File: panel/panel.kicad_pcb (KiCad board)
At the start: 2 copper layers, 40 x 40 mm, 0 parts

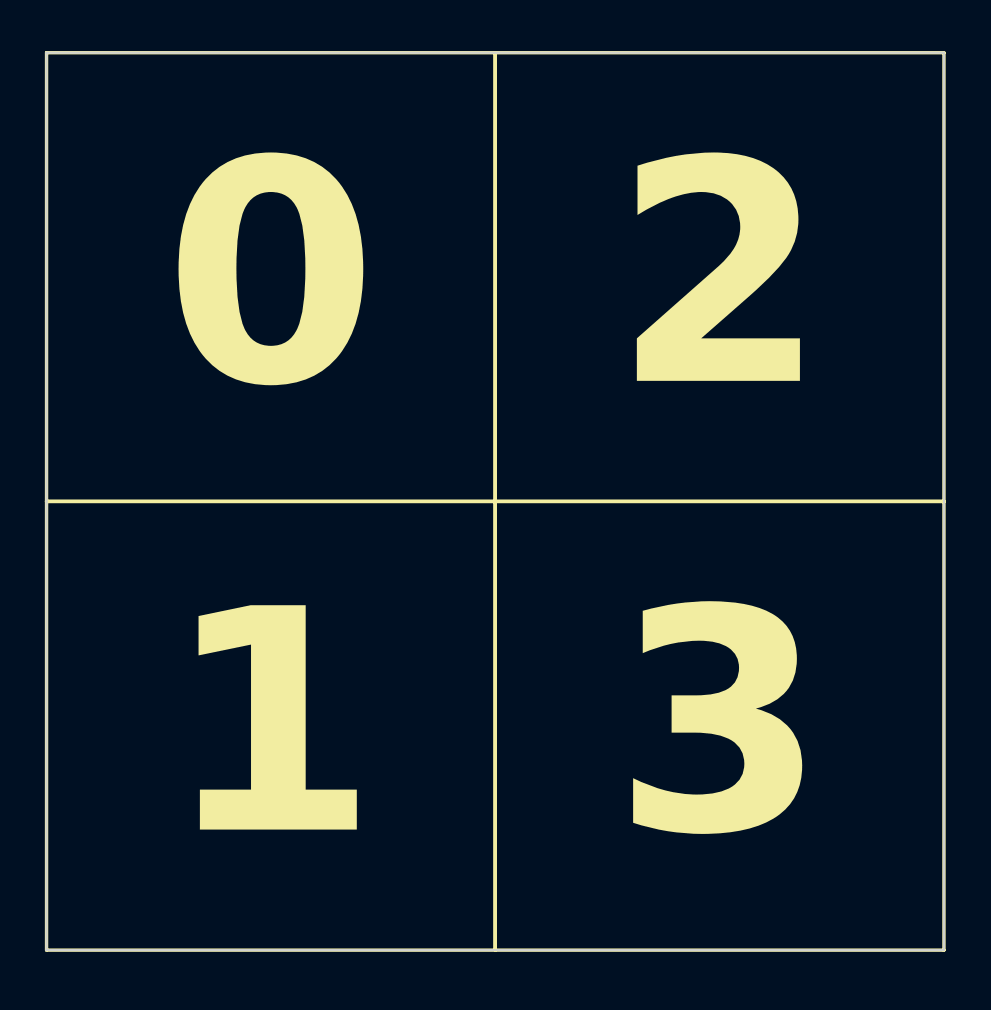
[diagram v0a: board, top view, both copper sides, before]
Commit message: Update panel
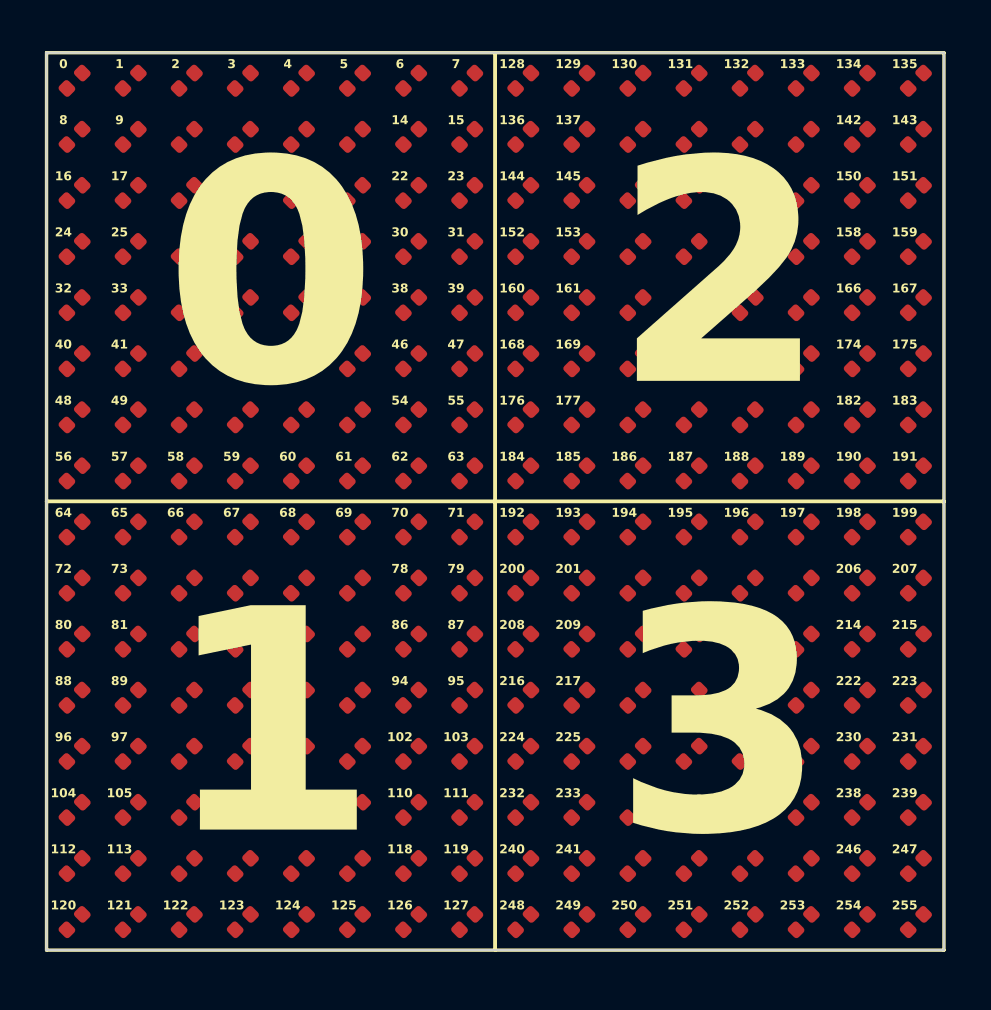
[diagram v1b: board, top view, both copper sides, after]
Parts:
- added REF**: LED_0402_1005Metric, LED_SMD:LED_0402_1005Metric, F.Cu at (146.2, 91.2)
- added REF**: LED_0402_1005Metric, LED_SMD:LED_0402_1005Metric, F.Cu at (138.8, 96.2)
- added REF**: LED_0402_1005Metric, LED_SMD:LED_0402_1005Metric, F.Cu at (116.2, 128.8)
- added REF**: LED_0402_1005Metric, LED_SMD:LED_0402_1005Metric, F.Cu at (116.2, 101.2)
- added REF**: LED_0402_1005Metric, LED_SMD:LED_0402_1005Metric, F.Cu at (153.8, 126.2)
- added REF**: LED_0402_1005Metric, LED_SMD:LED_0402_1005Metric, F.Cu at (151.2, 96.2)
- added REF**: LED_0402_1005Metric, LED_SMD:LED_0402_1005Metric, F.Cu at (118.8, 111.2)
- added REF**: LED_0402_1005Metric, LED_SMD:LED_0402_1005Metric, F.Cu at (128.8, 106.2)
- added REF**: LED_0402_1005Metric, LED_SMD:LED_0402_1005Metric, F.Cu at (131.2, 106.2)
- added REF**: LED_0402_1005Metric, LED_SMD:LED_0402_1005Metric, F.Cu at (116.2, 91.2)
- added REF**: LED_0402_1005Metric, LED_SMD:LED_0402_1005Metric, F.Cu at (128.8, 103.8)
- added REF**: LED_0402_1005Metric, LED_SMD:LED_0402_1005Metric, F.Cu at (138.8, 103.8)
- added REF**: LED_0402_1005Metric, LED_SMD:LED_0402_1005Metric, F.Cu at (126.2, 113.8)
- added REF**: LED_0402_1005Metric, LED_SMD:LED_0402_1005Metric, F.Cu at (121.2, 91.2)
- added REF**: LED_0402_1005Metric, LED_SMD:LED_0402_1005Metric, F.Cu at (138.8, 121.2)
- added REF**: LED_0402_1005Metric, LED_SMD:LED_0402_1005Metric, F.Cu at (136.2, 96.2)
- added REF**: LED_0402_1005Metric, LED_SMD:LED_0402_1005Metric, F.Cu at (153.8, 96.2)
- added REF**: LED_0402_1005Metric, LED_SMD:LED_0402_1005Metric, F.Cu at (153.8, 93.8)
- added REF**: LED_0402_1005Metric, LED_SMD:LED_0402_1005Metric, F.Cu at (148.8, 118.8)
- added REF**: LED_0402_1005Metric, LED_SMD:LED_0402_1005Metric, F.Cu at (138.8, 111.2)
- added REF**: LED_0402_1005Metric, LED_SMD:LED_0402_1005Metric, F.Cu at (118.8, 106.2)
- added REF**: LED_0402_1005Metric, LED_SMD:LED_0402_1005Metric, F.Cu at (116.2, 106.2)
- added REF**: LED_0402_1005Metric, LED_SMD:LED_0402_1005Metric, F.Cu at (131.2, 118.8)
- added REF**: LED_0402_1005Metric, LED_SMD:LED_0402_1005Metric, F.Cu at (136.2, 106.2)
- added REF**: LED_0402_1005Metric, LED_SMD:LED_0402_1005Metric, F.Cu at (128.8, 108.8)
- added REF**: LED_0402_1005Metric, LED_SMD:LED_0402_1005Metric, F.Cu at (143.8, 91.2)
- added REF**: LED_0402_1005Metric, LED_SMD:LED_0402_1005Metric, F.Cu at (128.8, 126.2)
- added REF**: LED_0402_1005Metric, LED_SMD:LED_0402_1005Metric, F.Cu at (126.2, 121.2)
- added REF**: LED_0402_1005Metric, LED_SMD:LED_0402_1005Metric, F.Cu at (131.2, 123.8)
- added REF**: LED_0402_1005Metric, LED_SMD:LED_0402_1005Metric, F.Cu at (148.8, 123.8)
- added REF**: LED_0402_1005Metric, LED_SMD:LED_0402_1005Metric, F.Cu at (131.2, 116.2)
- added REF**: LED_0402_1005Metric, LED_SMD:LED_0402_1005Metric, F.Cu at (141.2, 126.2)
- added REF**: LED_0402_1005Metric, LED_SMD:LED_0402_1005Metric, F.Cu at (128.8, 93.8)
- added REF**: LED_0402_1005Metric, LED_SMD:LED_0402_1005Metric, F.Cu at (136.2, 101.2)
- added REF**: LED_0402_1005Metric, LED_SMD:LED_0402_1005Metric, F.Cu at (131.2, 93.8)
- added REF**: LED_0402_1005Metric, LED_SMD:LED_0402_1005Metric, F.Cu at (128.8, 91.2)
- added REF**: LED_0402_1005Metric, LED_SMD:LED_0402_1005Metric, F.Cu at (118.8, 118.8)
- added REF**: LED_0402_1005Metric, LED_SMD:LED_0402_1005Metric, F.Cu at (128.8, 123.8)
- added REF**: LED_0402_1005Metric, LED_SMD:LED_0402_1005Metric, F.Cu at (136.2, 128.8)
- added REF**: LED_0402_1005Metric, LED_SMD:LED_0402_1005Metric, F.Cu at (116.2, 93.8)
- added REF**: LED_0402_1005Metric, LED_SMD:LED_0402_1005Metric, F.Cu at (133.8, 121.2)
- added REF**: LED_0402_1005Metric, LED_SMD:LED_0402_1005Metric, F.Cu at (123.8, 116.2)
- added REF**: LED_0402_1005Metric, LED_SMD:LED_0402_1005Metric, F.Cu at (118.8, 121.2)
- added REF**: LED_0402_1005Metric, LED_SMD:LED_0402_1005Metric, F.Cu at (126.2, 118.8)
- added REF**: LED_0402_1005Metric, LED_SMD:LED_0402_1005Metric, F.Cu at (148.8, 101.2)
- added REF**: LED_0402_1005Metric, LED_SMD:LED_0402_1005Metric, F.Cu at (118.8, 91.2)
- added REF**: LED_0402_1005Metric, LED_SMD:LED_0402_1005Metric, F.Cu at (141.2, 101.2)
- added REF**: LED_0402_1005Metric, LED_SMD:LED_0402_1005Metric, F.Cu at (143.8, 121.2)
- added REF**: LED_0402_1005Metric, LED_SMD:LED_0402_1005Metric, F.Cu at (128.8, 101.2)
- added REF**: LED_0402_1005Metric, LED_SMD:LED_0402_1005Metric, F.Cu at (143.8, 111.2)
- added REF**: LED_0402_1005Metric, LED_SMD:LED_0402_1005Metric, F.Cu at (148.8, 108.8)
- added REF**: LED_0402_1005Metric, LED_SMD:LED_0402_1005Metric, F.Cu at (121.2, 116.2)
- added REF**: LED_0402_1005Metric, LED_SMD:LED_0402_1005Metric, F.Cu at (153.8, 121.2)
- added REF**: LED_0402_1005Metric, LED_SMD:LED_0402_1005Metric, F.Cu at (126.2, 93.8)
- added REF**: LED_0402_1005Metric, LED_SMD:LED_0402_1005Metric, F.Cu at (118.8, 93.8)
- added REF**: LED_0402_1005Metric, LED_SMD:LED_0402_1005Metric, F.Cu at (143.8, 128.8)
- added REF**: LED_0402_1005Metric, LED_SMD:LED_0402_1005Metric, F.Cu at (133.8, 108.8)
- added REF**: LED_0402_1005Metric, LED_SMD:LED_0402_1005Metric, F.Cu at (138.8, 123.8)
- added REF**: LED_0402_1005Metric, LED_SMD:LED_0402_1005Metric, F.Cu at (123.8, 103.8)
- added REF**: LED_0402_1005Metric, LED_SMD:LED_0402_1005Metric, F.Cu at (138.8, 128.8)
- added REF**: LED_0402_1005Metric, LED_SMD:LED_0402_1005Metric, F.Cu at (131.2, 98.8)
- added REF**: LED_0402_1005Metric, LED_SMD:LED_0402_1005Metric, F.Cu at (126.2, 111.2)
- added REF**: LED_0402_1005Metric, LED_SMD:LED_0402_1005Metric, F.Cu at (153.8, 111.2)
- added REF**: LED_0402_1005Metric, LED_SMD:LED_0402_1005Metric, F.Cu at (153.8, 113.8)
- added REF**: LED_0402_1005Metric, LED_SMD:LED_0402_1005Metric, F.Cu at (148.8, 126.2)
- added REF**: LED_0402_1005Metric, LED_SMD:LED_0402_1005Metric, F.Cu at (133.8, 103.8)
- added REF**: LED_0402_1005Metric, LED_SMD:LED_0402_1005Metric, F.Cu at (133.8, 96.2)
- added REF**: LED_0402_1005Metric, LED_SMD:LED_0402_1005Metric, F.Cu at (131.2, 108.8)
- added REF**: LED_0402_1005Metric, LED_SMD:LED_0402_1005Metric, F.Cu at (136.2, 111.2)
- added REF**: LED_0402_1005Metric, LED_SMD:LED_0402_1005Metric, F.Cu at (121.2, 113.8)
- added REF**: LED_0402_1005Metric, LED_SMD:LED_0402_1005Metric, F.Cu at (141.2, 106.2)
- added REF**: LED_0402_1005Metric, LED_SMD:LED_0402_1005Metric, F.Cu at (128.8, 128.8)
- added REF**: LED_0402_1005Metric, LED_SMD:LED_0402_1005Metric, F.Cu at (146.2, 103.8)
- added REF**: LED_0402_1005Metric, LED_SMD:LED_0402_1005Metric, F.Cu at (141.2, 121.2)
- added REF**: LED_0402_1005Metric, LED_SMD:LED_0402_1005Metric, F.Cu at (146.2, 106.2)
- added REF**: LED_0402_1005Metric, LED_SMD:LED_0402_1005Metric, F.Cu at (153.8, 123.8)
- added REF**: LED_0402_1005Metric, LED_SMD:LED_0402_1005Metric, F.Cu at (118.8, 113.8)
- added REF**: LED_0402_1005Metric, LED_SMD:LED_0402_1005Metric, F.Cu at (153.8, 98.8)
- added REF**: LED_0402_1005Metric, LED_SMD:LED_0402_1005Metric, F.Cu at (143.8, 98.8)
- added REF**: LED_0402_1005Metric, LED_SMD:LED_0402_1005Metric, F.Cu at (116.2, 96.2)
- added REF**: LED_0402_1005Metric, LED_SMD:LED_0402_1005Metric, F.Cu at (138.8, 98.8)
- added REF**: LED_0402_1005Metric, LED_SMD:LED_0402_1005Metric, F.Cu at (118.8, 116.2)
- added REF**: LED_0402_1005Metric, LED_SMD:LED_0402_1005Metric, F.Cu at (143.8, 103.8)
- added REF**: LED_0402_1005Metric, LED_SMD:LED_0402_1005Metric, F.Cu at (126.2, 128.8)
- added REF**: LED_0402_1005Metric, LED_SMD:LED_0402_1005Metric, F.Cu at (138.8, 113.8)
- added REF**: LED_0402_1005Metric, LED_SMD:LED_0402_1005Metric, F.Cu at (133.8, 113.8)
- added REF**: LED_0402_1005Metric, LED_SMD:LED_0402_1005Metric, F.Cu at (118.8, 101.2)
- added REF**: LED_0402_1005Metric, LED_SMD:LED_0402_1005Metric, F.Cu at (138.8, 93.8)
- added REF**: LED_0402_1005Metric, LED_SMD:LED_0402_1005Metric, F.Cu at (131.2, 113.8)
- added REF**: LED_0402_1005Metric, LED_SMD:LED_0402_1005Metric, F.Cu at (116.2, 111.2)
- added REF**: LED_0402_1005Metric, LED_SMD:LED_0402_1005Metric, F.Cu at (126.2, 96.2)
- added REF**: LED_0402_1005Metric, LED_SMD:LED_0402_1005Metric, F.Cu at (118.8, 108.8)
- added REF**: LED_0402_1005Metric, LED_SMD:LED_0402_1005Metric, F.Cu at (126.2, 116.2)
- added REF**: LED_0402_1005Metric, LED_SMD:LED_0402_1005Metric, F.Cu at (143.8, 106.2)
- added REF**: LED_0402_1005Metric, LED_SMD:LED_0402_1005Metric, F.Cu at (116.2, 108.8)
- added REF**: LED_0402_1005Metric, LED_SMD:LED_0402_1005Metric, F.Cu at (136.2, 121.2)
- added REF**: LED_0402_1005Metric, LED_SMD:LED_0402_1005Metric, F.Cu at (121.2, 103.8)
- added REF**: LED_0402_1005Metric, LED_SMD:LED_0402_1005Metric, F.Cu at (138.8, 108.8)
- added REF**: LED_0402_1005Metric, LED_SMD:LED_0402_1005Metric, F.Cu at (133.8, 93.8)
- added REF**: LED_0402_1005Metric, LED_SMD:LED_0402_1005Metric, F.Cu at (148.8, 93.8)
- added REF**: LED_0402_1005Metric, LED_SMD:LED_0402_1005Metric, F.Cu at (116.2, 126.2)
- added REF**: LED_0402_1005Metric, LED_SMD:LED_0402_1005Metric, F.Cu at (146.2, 101.2)
- added REF**: LED_0402_1005Metric, LED_SMD:LED_0402_1005Metric, F.Cu at (123.8, 123.8)
- added REF**: LED_0402_1005Metric, LED_SMD:LED_0402_1005Metric, F.Cu at (121.2, 126.2)
- added REF**: LED_0402_1005Metric, LED_SMD:LED_0402_1005Metric, F.Cu at (148.8, 116.2)
- added REF**: LED_0402_1005Metric, LED_SMD:LED_0402_1005Metric, F.Cu at (116.2, 123.8)
- added REF**: LED_0402_1005Metric, LED_SMD:LED_0402_1005Metric, F.Cu at (131.2, 126.2)
- added REF**: LED_0402_1005Metric, LED_SMD:LED_0402_1005Metric, F.Cu at (131.2, 96.2)
- added REF**: LED_0402_1005Metric, LED_SMD:LED_0402_1005Metric, F.Cu at (118.8, 123.8)
- added REF**: LED_0402_1005Metric, LED_SMD:LED_0402_1005Metric, F.Cu at (138.8, 106.2)
- added REF**: LED_0402_1005Metric, LED_SMD:LED_0402_1005Metric, F.Cu at (141.2, 96.2)
- added REF**: LED_0402_1005Metric, LED_SMD:LED_0402_1005Metric, F.Cu at (153.8, 116.2)
- added REF**: LED_0402_1005Metric, LED_SMD:LED_0402_1005Metric, F.Cu at (118.8, 126.2)
- added REF**: LED_0402_1005Metric, LED_SMD:LED_0402_1005Metric, F.Cu at (151.2, 123.8)
- added REF**: LED_0402_1005Metric, LED_SMD:LED_0402_1005Metric, F.Cu at (133.8, 128.8)
- added REF**: LED_0402_1005Metric, LED_SMD:LED_0402_1005Metric, F.Cu at (143.8, 116.2)
- added REF**: LED_0402_1005Metric, LED_SMD:LED_0402_1005Metric, F.Cu at (128.8, 98.8)
- added REF**: LED_0402_1005Metric, LED_SMD:LED_0402_1005Metric, F.Cu at (141.2, 118.8)
- added REF**: LED_0402_1005Metric, LED_SMD:LED_0402_1005Metric, F.Cu at (148.8, 121.2)
- added REF**: LED_0402_1005Metric, LED_SMD:LED_0402_1005Metric, F.Cu at (141.2, 116.2)
- added REF**: LED_0402_1005Metric, LED_SMD:LED_0402_1005Metric, F.Cu at (141.2, 98.8)
- added REF**: LED_0402_1005Metric, LED_SMD:LED_0402_1005Metric, F.Cu at (136.2, 126.2)
- added REF**: LED_0402_1005Metric, LED_SMD:LED_0402_1005Metric, F.Cu at (136.2, 108.8)
- added REF**: LED_0402_1005Metric, LED_SMD:LED_0402_1005Metric, F.Cu at (116.2, 121.2)
- added REF**: LED_0402_1005Metric, LED_SMD:LED_0402_1005Metric, F.Cu at (141.2, 111.2)
- added REF**: LED_0402_1005Metric, LED_SMD:LED_0402_1005Metric, F.Cu at (126.2, 103.8)
- added REF**: LED_0402_1005Metric, LED_SMD:LED_0402_1005Metric, F.Cu at (146.2, 108.8)
- added REF**: LED_0402_1005Metric, LED_SMD:LED_0402_1005Metric, F.Cu at (143.8, 113.8)
- added REF**: LED_0402_1005Metric, LED_SMD:LED_0402_1005Metric, F.Cu at (146.2, 126.2)
- added REF**: LED_0402_1005Metric, LED_SMD:LED_0402_1005Metric, F.Cu at (121.2, 108.8)
- added REF**: LED_0402_1005Metric, LED_SMD:LED_0402_1005Metric, F.Cu at (126.2, 123.8)
- added REF**: LED_0402_1005Metric, LED_SMD:LED_0402_1005Metric, F.Cu at (123.8, 106.2)
- added REF**: LED_0402_1005Metric, LED_SMD:LED_0402_1005Metric, F.Cu at (121.2, 118.8)
- added REF**: LED_0402_1005Metric, LED_SMD:LED_0402_1005Metric, F.Cu at (131.2, 101.2)
- added REF**: LED_0402_1005Metric, LED_SMD:LED_0402_1005Metric, F.Cu at (131.2, 111.2)
- added REF**: LED_0402_1005Metric, LED_SMD:LED_0402_1005Metric, F.Cu at (126.2, 106.2)
- added REF**: LED_0402_1005Metric, LED_SMD:LED_0402_1005Metric, F.Cu at (128.8, 96.2)
- added REF**: LED_0402_1005Metric, LED_SMD:LED_0402_1005Metric, F.Cu at (136.2, 103.8)
- added REF**: LED_0402_1005Metric, LED_SMD:LED_0402_1005Metric, F.Cu at (126.2, 108.8)
- added REF**: LED_0402_1005Metric, LED_SMD:LED_0402_1005Metric, F.Cu at (153.8, 106.2)
- added REF**: LED_0402_1005Metric, LED_SMD:LED_0402_1005Metric, F.Cu at (143.8, 93.8)
- added REF**: LED_0402_1005Metric, LED_SMD:LED_0402_1005Metric, F.Cu at (118.8, 96.2)
- added REF**: LED_0402_1005Metric, LED_SMD:LED_0402_1005Metric, F.Cu at (151.2, 113.8)
- added REF**: LED_0402_1005Metric, LED_SMD:LED_0402_1005Metric, F.Cu at (146.2, 123.8)
- added REF**: LED_0402_1005Metric, LED_SMD:LED_0402_1005Metric, F.Cu at (151.2, 101.2)
- added REF**: LED_0402_1005Metric, LED_SMD:LED_0402_1005Metric, F.Cu at (141.2, 123.8)
- added REF**: LED_0402_1005Metric, LED_SMD:LED_0402_1005Metric, F.Cu at (128.8, 116.2)
- added REF**: LED_0402_1005Metric, LED_SMD:LED_0402_1005Metric, F.Cu at (153.8, 128.8)
- added REF**: LED_0402_1005Metric, LED_SMD:LED_0402_1005Metric, F.Cu at (151.2, 108.8)
- added REF**: LED_0402_1005Metric, LED_SMD:LED_0402_1005Metric, F.Cu at (133.8, 91.2)
- added REF**: LED_0402_1005Metric, LED_SMD:LED_0402_1005Metric, F.Cu at (148.8, 111.2)
- added REF**: LED_0402_1005Metric, LED_SMD:LED_0402_1005Metric, F.Cu at (148.8, 128.8)
- added REF**: LED_0402_1005Metric, LED_SMD:LED_0402_1005Metric, F.Cu at (153.8, 91.2)
- added REF**: LED_0402_1005Metric, LED_SMD:LED_0402_1005Metric, F.Cu at (148.8, 106.2)
- added REF**: LED_0402_1005Metric, LED_SMD:LED_0402_1005Metric, F.Cu at (143.8, 123.8)
- added REF**: LED_0402_1005Metric, LED_SMD:LED_0402_1005Metric, F.Cu at (141.2, 113.8)
- added REF**: LED_0402_1005Metric, LED_SMD:LED_0402_1005Metric, F.Cu at (126.2, 98.8)
- added REF**: LED_0402_1005Metric, LED_SMD:LED_0402_1005Metric, F.Cu at (131.2, 103.8)
- added REF**: LED_0402_1005Metric, LED_SMD:LED_0402_1005Metric, F.Cu at (116.2, 103.8)
- added REF**: LED_0402_1005Metric, LED_SMD:LED_0402_1005Metric, F.Cu at (123.8, 91.2)
- added REF**: LED_0402_1005Metric, LED_SMD:LED_0402_1005Metric, F.Cu at (116.2, 116.2)
- added REF**: LED_0402_1005Metric, LED_SMD:LED_0402_1005Metric, F.Cu at (138.8, 126.2)
- added REF**: LED_0402_1005Metric, LED_SMD:LED_0402_1005Metric, F.Cu at (146.2, 98.8)
- added REF**: LED_0402_1005Metric, LED_SMD:LED_0402_1005Metric, F.Cu at (136.2, 118.8)
- added REF**: LED_0402_1005Metric, LED_SMD:LED_0402_1005Metric, F.Cu at (148.8, 113.8)
- added REF**: LED_0402_1005Metric, LED_SMD:LED_0402_1005Metric, F.Cu at (151.2, 128.8)
- added REF**: LED_0402_1005Metric, LED_SMD:LED_0402_1005Metric, F.Cu at (136.2, 98.8)
- added REF**: LED_0402_1005Metric, LED_SMD:LED_0402_1005Metric, F.Cu at (123.8, 101.2)
- added REF**: LED_0402_1005Metric, LED_SMD:LED_0402_1005Metric, F.Cu at (136.2, 116.2)
- added REF**: LED_0402_1005Metric, LED_SMD:LED_0402_1005Metric, F.Cu at (153.8, 108.8)
- added REF**: LED_0402_1005Metric, LED_SMD:LED_0402_1005Metric, F.Cu at (146.2, 116.2)
- added REF**: LED_0402_1005Metric, LED_SMD:LED_0402_1005Metric, F.Cu at (138.8, 101.2)
- added REF**: LED_0402_1005Metric, LED_SMD:LED_0402_1005Metric, F.Cu at (153.8, 118.8)
- added REF**: LED_0402_1005Metric, LED_SMD:LED_0402_1005Metric, F.Cu at (123.8, 111.2)
- added REF**: LED_0402_1005Metric, LED_SMD:LED_0402_1005Metric, F.Cu at (146.2, 93.8)
- added REF**: LED_0402_1005Metric, LED_SMD:LED_0402_1005Metric, F.Cu at (136.2, 91.2)
- added REF**: LED_0402_1005Metric, LED_SMD:LED_0402_1005Metric, F.Cu at (118.8, 98.8)
- added REF**: LED_0402_1005Metric, LED_SMD:LED_0402_1005Metric, F.Cu at (123.8, 96.2)
- added REF**: LED_0402_1005Metric, LED_SMD:LED_0402_1005Metric, F.Cu at (148.8, 91.2)
- added REF**: LED_0402_1005Metric, LED_SMD:LED_0402_1005Metric, F.Cu at (143.8, 96.2)
- added REF**: LED_0402_1005Metric, LED_SMD:LED_0402_1005Metric, F.Cu at (133.8, 111.2)
- added REF**: LED_0402_1005Metric, LED_SMD:LED_0402_1005Metric, F.Cu at (146.2, 113.8)
- added REF**: LED_0402_1005Metric, LED_SMD:LED_0402_1005Metric, F.Cu at (151.2, 91.2)
- added REF**: LED_0402_1005Metric, LED_SMD:LED_0402_1005Metric, F.Cu at (143.8, 101.2)
- added REF**: LED_0402_1005Metric, LED_SMD:LED_0402_1005Metric, F.Cu at (133.8, 106.2)
- added REF**: LED_0402_1005Metric, LED_SMD:LED_0402_1005Metric, F.Cu at (123.8, 121.2)
- added REF**: LED_0402_1005Metric, LED_SMD:LED_0402_1005Metric, F.Cu at (121.2, 93.8)
- added REF**: LED_0402_1005Metric, LED_SMD:LED_0402_1005Metric, F.Cu at (128.8, 111.2)
- added REF**: LED_0402_1005Metric, LED_SMD:LED_0402_1005Metric, F.Cu at (151.2, 118.8)
- added REF**: LED_0402_1005Metric, LED_SMD:LED_0402_1005Metric, F.Cu at (143.8, 118.8)
- added REF**: LED_0402_1005Metric, LED_SMD:LED_0402_1005Metric, F.Cu at (136.2, 113.8)
- added REF**: LED_0402_1005Metric, LED_SMD:LED_0402_1005Metric, F.Cu at (123.8, 113.8)
- added REF**: LED_0402_1005Metric, LED_SMD:LED_0402_1005Metric, F.Cu at (121.2, 123.8)
- added REF**: LED_0402_1005Metric, LED_SMD:LED_0402_1005Metric, F.Cu at (126.2, 91.2)
- added REF**: LED_0402_1005Metric, LED_SMD:LED_0402_1005Metric, F.Cu at (138.8, 91.2)
- added REF**: LED_0402_1005Metric, LED_SMD:LED_0402_1005Metric, F.Cu at (151.2, 98.8)
- added REF**: LED_0402_1005Metric, LED_SMD:LED_0402_1005Metric, F.Cu at (133.8, 118.8)
- added REF**: LED_0402_1005Metric, LED_SMD:LED_0402_1005Metric, F.Cu at (116.2, 118.8)
- added REF**: LED_0402_1005Metric, LED_SMD:LED_0402_1005Metric, F.Cu at (136.2, 93.8)
- added REF**: LED_0402_1005Metric, LED_SMD:LED_0402_1005Metric, F.Cu at (138.8, 118.8)
- added REF**: LED_0402_1005Metric, LED_SMD:LED_0402_1005Metric, F.Cu at (123.8, 128.8)
- added REF**: LED_0402_1005Metric, LED_SMD:LED_0402_1005Metric, F.Cu at (123.8, 98.8)
- added REF**: LED_0402_1005Metric, LED_SMD:LED_0402_1005Metric, F.Cu at (123.8, 126.2)
- added REF**: LED_0402_1005Metric, LED_SMD:LED_0402_1005Metric, F.Cu at (131.2, 121.2)
- added REF**: LED_0402_1005Metric, LED_SMD:LED_0402_1005Metric, F.Cu at (133.8, 116.2)
- added REF**: LED_0402_1005Metric, LED_SMD:LED_0402_1005Metric, F.Cu at (121.2, 121.2)
- added REF**: LED_0402_1005Metric, LED_SMD:LED_0402_1005Metric, F.Cu at (133.8, 101.2)
- added REF**: LED_0402_1005Metric, LED_SMD:LED_0402_1005Metric, F.Cu at (133.8, 126.2)
- added REF**: LED_0402_1005Metric, LED_SMD:LED_0402_1005Metric, F.Cu at (116.2, 98.8)
- added REF**: LED_0402_1005Metric, LED_SMD:LED_0402_1005Metric, F.Cu at (141.2, 93.8)
- added REF**: LED_0402_1005Metric, LED_SMD:LED_0402_1005Metric, F.Cu at (141.2, 103.8)
- added REF**: LED_0402_1005Metric, LED_SMD:LED_0402_1005Metric, F.Cu at (133.8, 123.8)
- added REF**: LED_0402_1005Metric, LED_SMD:LED_0402_1005Metric, F.Cu at (148.8, 98.8)
- added REF**: LED_0402_1005Metric, LED_SMD:LED_0402_1005Metric, F.Cu at (118.8, 103.8)
- added REF**: LED_0402_1005Metric, LED_SMD:LED_0402_1005Metric, F.Cu at (121.2, 128.8)
- added REF**: LED_0402_1005Metric, LED_SMD:LED_0402_1005Metric, F.Cu at (121.2, 111.2)
- added REF**: LED_0402_1005Metric, LED_SMD:LED_0402_1005Metric, F.Cu at (143.8, 108.8)
- added REF**: LED_0402_1005Metric, LED_SMD:LED_0402_1005Metric, F.Cu at (128.8, 118.8)
- added REF**: LED_0402_1005Metric, LED_SMD:LED_0402_1005Metric, F.Cu at (131.2, 128.8)
- added REF**: LED_0402_1005Metric, LED_SMD:LED_0402_1005Metric, F.Cu at (136.2, 123.8)
- added REF**: LED_0402_1005Metric, LED_SMD:LED_0402_1005Metric, F.Cu at (146.2, 96.2)
- added REF**: LED_0402_1005Metric, LED_SMD:LED_0402_1005Metric, F.Cu at (118.8, 128.8)
- added REF**: LED_0402_1005Metric, LED_SMD:LED_0402_1005Metric, F.Cu at (133.8, 98.8)
- added REF**: LED_0402_1005Metric, LED_SMD:LED_0402_1005Metric, F.Cu at (151.2, 103.8)
- added REF**: LED_0402_1005Metric, LED_SMD:LED_0402_1005Metric, F.Cu at (121.2, 96.2)
- added REF**: LED_0402_1005Metric, LED_SMD:LED_0402_1005Metric, F.Cu at (141.2, 128.8)
- added REF**: LED_0402_1005Metric, LED_SMD:LED_0402_1005Metric, F.Cu at (138.8, 116.2)
- added REF**: LED_0402_1005Metric, LED_SMD:LED_0402_1005Metric, F.Cu at (146.2, 128.8)
- added REF**: LED_0402_1005Metric, LED_SMD:LED_0402_1005Metric, F.Cu at (151.2, 93.8)
- added REF**: LED_0402_1005Metric, LED_SMD:LED_0402_1005Metric, F.Cu at (123.8, 118.8)
- added REF**: LED_0402_1005Metric, LED_SMD:LED_0402_1005Metric, F.Cu at (141.2, 108.8)
- added REF**: LED_0402_1005Metric, LED_SMD:LED_0402_1005Metric, F.Cu at (121.2, 101.2)
- added REF**: LED_0402_1005Metric, LED_SMD:LED_0402_1005Metric, F.Cu at (121.2, 98.8)
- added REF**: LED_0402_1005Metric, LED_SMD:LED_0402_1005Metric, F.Cu at (153.8, 101.2)
- added REF**: LED_0402_1005Metric, LED_SMD:LED_0402_1005Metric, F.Cu at (128.8, 113.8)
- added REF**: LED_0402_1005Metric, LED_SMD:LED_0402_1005Metric, F.Cu at (151.2, 111.2)
- added REF**: LED_0402_1005Metric, LED_SMD:LED_0402_1005Metric, F.Cu at (128.8, 121.2)
- added REF**: LED_0402_1005Metric, LED_SMD:LED_0402_1005Metric, F.Cu at (151.2, 126.2)
- added REF**: LED_0402_1005Metric, LED_SMD:LED_0402_1005Metric, F.Cu at (126.2, 101.2)
- added REF**: LED_0402_1005Metric, LED_SMD:LED_0402_1005Metric, F.Cu at (131.2, 91.2)
- added REF**: LED_0402_1005Metric, LED_SMD:LED_0402_1005Metric, F.Cu at (146.2, 111.2)
- added REF**: LED_0402_1005Metric, LED_SMD:LED_0402_1005Metric, F.Cu at (141.2, 91.2)
- added REF**: LED_0402_1005Metric, LED_SMD:LED_0402_1005Metric, F.Cu at (146.2, 121.2)
- added REF**: LED_0402_1005Metric, LED_SMD:LED_0402_1005Metric, F.Cu at (143.8, 126.2)
- added REF**: LED_0402_1005Metric, LED_SMD:LED_0402_1005Metric, F.Cu at (151.2, 106.2)
- added REF**: LED_0402_1005Metric, LED_SMD:LED_0402_1005Metric, F.Cu at (123.8, 108.8)
- added REF**: LED_0402_1005Metric, LED_SMD:LED_0402_1005Metric, F.Cu at (148.8, 96.2)
- added REF**: LED_0402_1005Metric, LED_SMD:LED_0402_1005Metric, F.Cu at (151.2, 121.2)
- added REF**: LED_0402_1005Metric, LED_SMD:LED_0402_1005Metric, F.Cu at (116.2, 113.8)
- added REF**: LED_0402_1005Metric, LED_SMD:LED_0402_1005Metric, F.Cu at (123.8, 93.8)
- added REF**: LED_0402_1005Metric, LED_SMD:LED_0402_1005Metric, F.Cu at (146.2, 118.8)
- added REF**: LED_0402_1005Metric, LED_SMD:LED_0402_1005Metric, F.Cu at (126.2, 126.2)
- added REF**: LED_0402_1005Metric, LED_SMD:LED_0402_1005Metric, F.Cu at (153.8, 103.8)
- added REF**: LED_0402_1005Metric, LED_SMD:LED_0402_1005Metric, F.Cu at (151.2, 116.2)
- added REF**: LED_0402_1005Metric, LED_SMD:LED_0402_1005Metric, F.Cu at (148.8, 103.8)
- added REF**: LED_0402_1005Metric, LED_SMD:LED_0402_1005Metric, F.Cu at (121.2, 106.2)
